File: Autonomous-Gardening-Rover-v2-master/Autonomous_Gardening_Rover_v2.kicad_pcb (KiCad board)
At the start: 6 copper layers, 60 parts, among them J1 Conn_01x05_Pin, J10 SENSORS, J11 Conn_01x02_Socket, J12 Conn_01x05_Pin, J14 Conn_01x05_Pin, J2 USB_B_Micro, J24 UWB SIGNAL, J3 Conn_01x05_Pin, J4 LINEAR ACTUATOR SIGNAL, J5 Screw_Terminal_01x02, J6 Screw_Terminal_01x02, J7 MPU SIGNAL, J8 Screw_Terminal_01x02, Q1 BC107, Q2 BC107, SW1 SW_Push, SW2 SW_Push, U1 ESP32-S3-WROOM-1, U2 CP2104, U3 LM358, U4 LM358, U6 MPU-6500

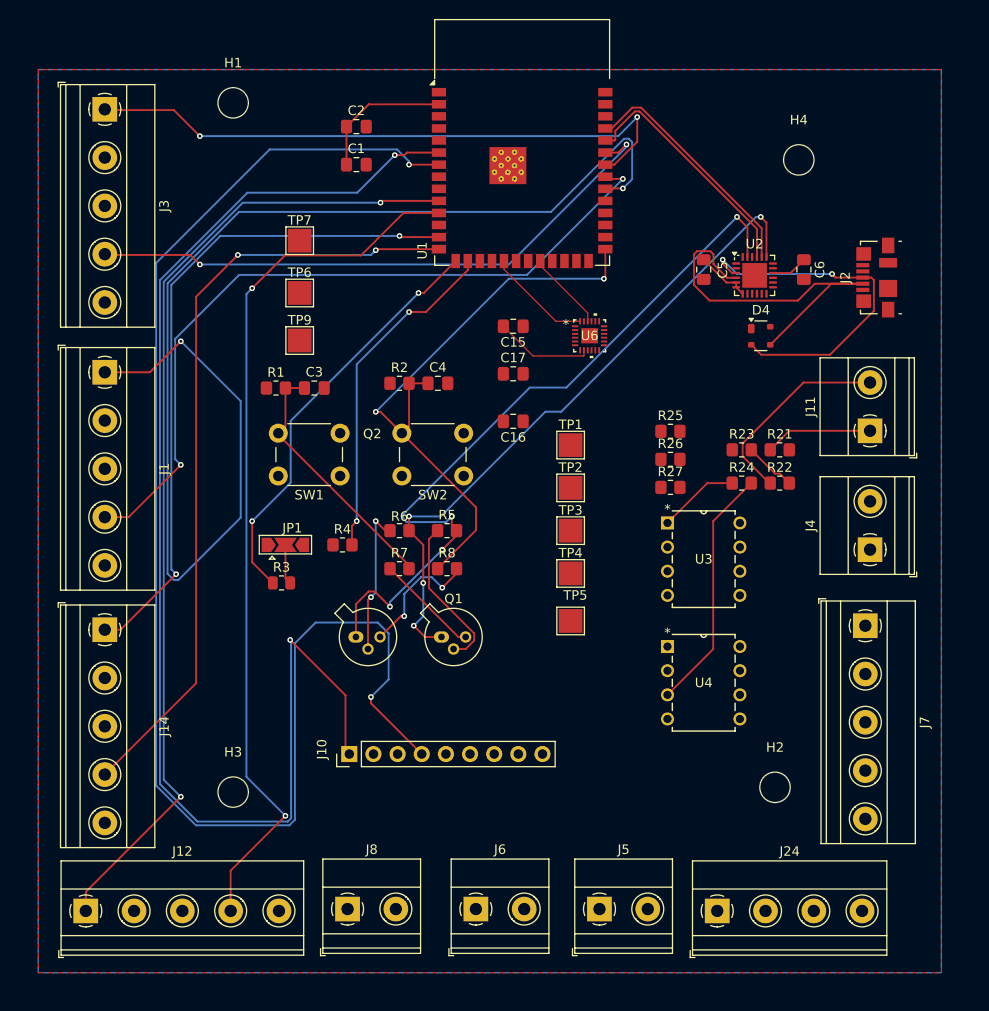
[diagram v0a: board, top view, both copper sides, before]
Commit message: Update PCB
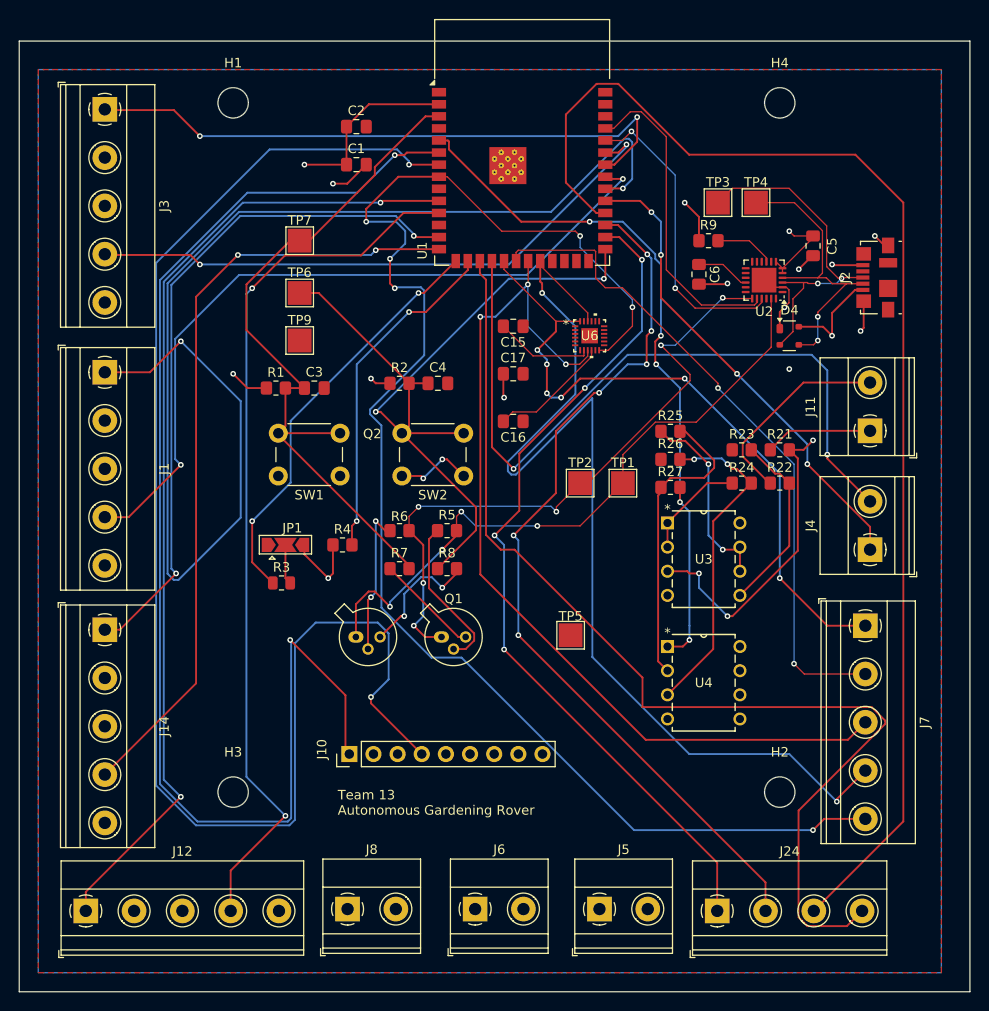
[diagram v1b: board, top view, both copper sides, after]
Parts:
- added R9: 4.7k, Resistor_SMD:R_0805_2012Metric_Pad1.20x1.40mm_HandSolder, F.Cu at (100.5, 53.0)
- moved TP4 43.6 mm to (105.5, 49.0)
- moved TP3 37.8 mm to (101.5, 49.0)
- moved C5 11.8 mm to (111.5, 53.5)
- moved C6 11.0 mm to (99.5, 56.5)
- moved TP1 6.80 mm to (91.5, 78.5)
- moved H4 6.32 mm to (108.0, 38.5)
- moved D4 3.00 mm to (109.0, 63.0)
- moved TP5 1.50 mm to (86.0, 94.5)
- moved TP2 1.12 mm to (87.0, 78.5)
- moved U2 1.12 mm to (106.3, 57.1), turned to 180 degrees
- moved H2 0.71 mm to (108.0, 111.0)
- moved J6 0.08 mm to (76.0, 123.3)
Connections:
- J2 pad 6: unconnected-(J2-Shield-Pad6) -> GND
- U2 pad 9: unconnected-(U2-~{RST}-Pad9) -> Net-(U2-~{RST})
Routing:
- net /MPUINT: track 0.00 -> 156.1 mm, vias 0 -> 6
- net /UWBMISO: track 0.00 -> 133.0 mm
- net /UWBCS: track 0.00 -> 113.2 mm
- net /MPUCS: track 8.40 -> 111.1 mm, vias 0 -> 2
- net /MPUMISO: track 0.00 -> 97.8 mm, vias 0 -> 3
- net /UWBCLK: track 0.00 -> 93.4 mm, vias 0 -> 6
- net /UWBMOSI: track 0.00 -> 89.5 mm, vias 0 -> 4
- net /LINACT-: track 0.00 -> 77.1 mm, vias 0 -> 2
- net /Moisture_Sensor_Output: track 0.00 -> 74.9 mm, vias 0 -> 5
- net /MPUCLK: track 0.00 -> 70.4 mm, vias 0 -> 2
- net +3V3: track 30.9 -> 93.4 mm, vias 0 -> 10
- net /MPUMOSI: track 11.1 -> 71.7 mm, vias 0 -> 6
- net /LINACT+: track 0.00 -> 50.4 mm, vias 0 -> 4
- net /CHIP_PU: track 27.0 -> 75.0 mm
- net GND: track 0.00 -> 33.5 mm, vias 0 -> 10
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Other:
- board outline added: 100 x 100 mm
- board text added: "Team 13 Autonomous Gardening Rover"
